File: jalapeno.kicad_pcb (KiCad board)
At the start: 2 copper layers, 230.1 x 77.6 mm, 187 parts, among them IC1 ATMEGA32U4-AU, J1 USB_B, J2 AVR-ISP-6, J3 Conn_01x04, K1 esc, K10 o, K11 p, K12 back, K13 tab, K14 a, K15 s, K16 d, K17 f, K18 g, K19 h, K2 q, K20 j, K21 k, K22 l, K23 ;, K24 caps, K25 caps, K26 z, K27 x, K28 c, K29 v, K3 w, K30 b, K31 n, K32 m, K33 ,, K33_1 ,, K34 ., K34_1 ., K35 ctrl, K36 gui, K37 alt, K37_1 alt, K38 space, K38_1 space, K39 alt, K39_1 gui, K4 e, K40 gui, K41 ctrl, K42 KEYSW, K5 r, K6 t, K7 y, K8 u, K9 i, Q1 MMBT2222ALT3G, SW1 SW_PUSH, U1 MDBT40, U2 SPX3819M5-L-3-3, U3 MCP73831T-2ACI/OT, Y1 XTAL_GND

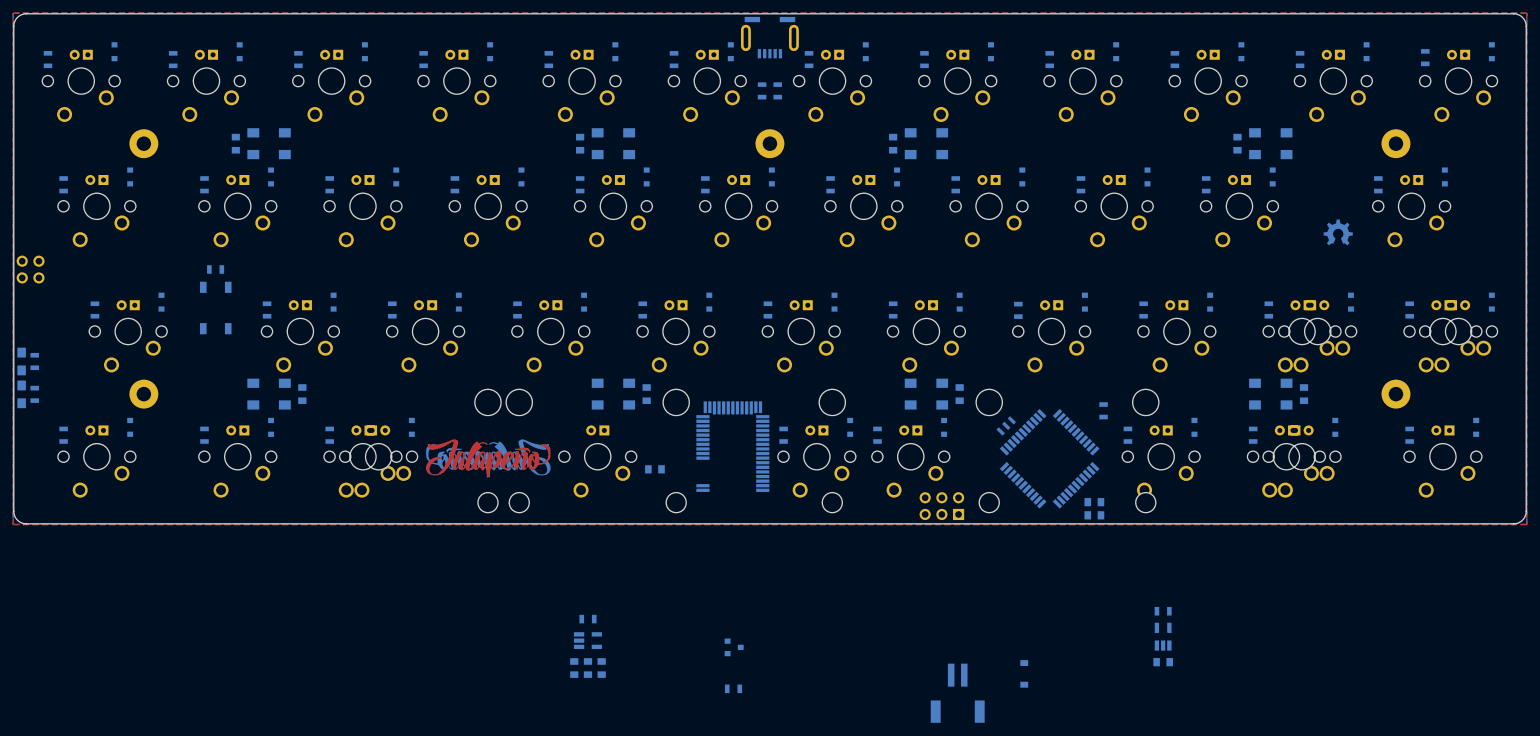
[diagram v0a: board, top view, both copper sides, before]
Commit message: routing + plate
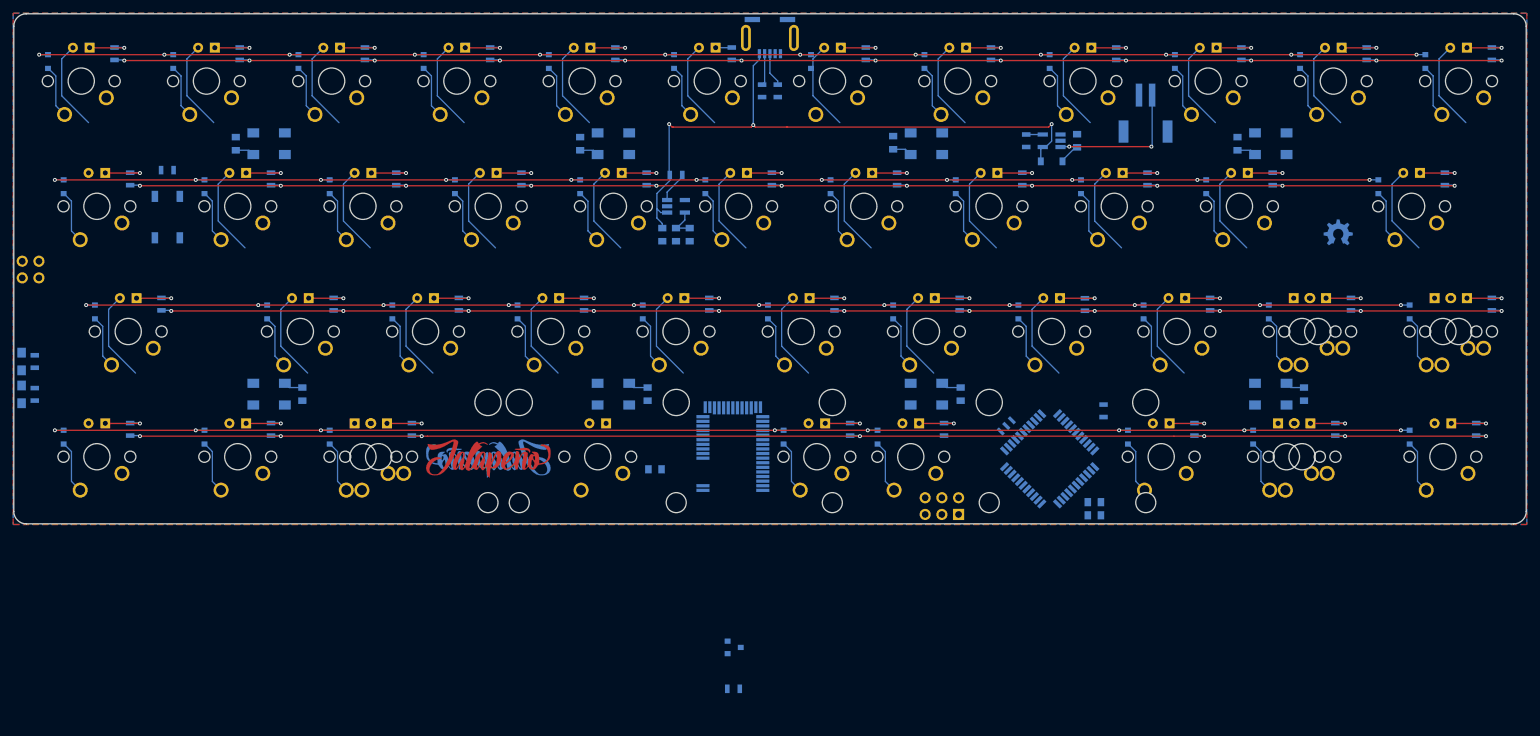
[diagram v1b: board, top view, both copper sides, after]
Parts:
- H1, H2, H3, H4, H6: footprint Mounting_Holes:MountingHole_2.2mm_M2_Pad -> Jalapeno:NOOP
- K33, K37_1: footprint Jalapeno:CHERRY_PCB_125H_LED_REVERSED -> Jalapeno:CHERRY_PCB_125H_LED
- K33_1, K37: footprint Jalapeno:CHERRY_PCB_100H_LED -> Jalapeno:CHERRY_PCB_100H_LED_REVERSED
- K34, K39_1: footprint Jalapeno:CHERRY_PCB_100H_LED_REVERSED -> Jalapeno:CHERRY_PCB_100H_LED
- K34_1, K39: footprint Jalapeno:CHERRY_PCB_125H_LED -> Jalapeno:CHERRY_PCB_125H_LED_REVERSED
- moved JST1 92.8 mm to (204.8, 42.7)
- moved C3 80.4 mm to (194.4, 42.4), turned to 90 degrees
- moved DB1 78.1 mm to (190.5, 45.5), turned to 0 degrees
- moved U3 77.3 mm to (190.5, 42.4), turned to 180 degrees
- moved R3 74.6 mm to (186.6, 42.4), turned to 90 degrees
- moved R6 68.9 mm to (133.3, 47.6)
- moved U2 67.4 mm to (133.3, 52.4)
- moved C5 67.3 mm to (133.3, 56.7)
- moved C6 67.3 mm to (131.3, 56.7)
- moved C7 67.3 mm to (135.4, 56.7)
- moved R7 16.8 mm to (56.0, 46.9), turned to 0 degrees
- moved SW1 15.7 mm to (56.0, 54.0), turned to 270 degrees
- moved D33 12.6 mm to (223.5, 68.5)
- moved D34 12.6 mm to (245.0, 68.5)
- moved D39 12.6 mm to (221.2, 87.5)
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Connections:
- K1 pad 1: COL_1 -> Net-(D1-Pad2)
- K1 pad 2: Net-(D1-Pad2) -> COL_1
- K10 pad 1: COL_10 -> Net-(D10-Pad2)
- K10 pad 2: Net-(D10-Pad2) -> COL_10
- K11 pad 1: COL_11 -> Net-(D11-Pad2)
- K11 pad 2: Net-(D11-Pad2) -> COL_11
- K12 pad 1: COL_12 -> Net-(D12-Pad2)
- K12 pad 2: Net-(D12-Pad2) -> COL_12
- K13 pad 1: COL_1 -> Net-(D13-Pad2)
- K13 pad 2: Net-(D13-Pad2) -> COL_1
- K14 pad 1: COL_2 -> Net-(D14-Pad2)
- K14 pad 2: Net-(D14-Pad2) -> COL_2
- K15 pad 1: COL_3 -> Net-(D15-Pad2)
- K15 pad 2: Net-(D15-Pad2) -> COL_3
- K16 pad 1: COL_4 -> Net-(D16-Pad2)
- K16 pad 2: Net-(D16-Pad2) -> COL_4
- K17 pad 1: COL_5 -> Net-(D17-Pad2)
- K17 pad 2: Net-(D17-Pad2) -> COL_5
- K18 pad 1: COL_6 -> Net-(D18-Pad2)
- K18 pad 2: Net-(D18-Pad2) -> COL_6
- K19 pad 1: COL_7 -> Net-(D19-Pad2)
- K19 pad 2: Net-(D19-Pad2) -> COL_7
- K2 pad 1: COL_2 -> Net-(D2-Pad2)
- K2 pad 2: Net-(D2-Pad2) -> COL_2
- K20 pad 1: COL_8 -> Net-(D20-Pad2)
- K20 pad 2: Net-(D20-Pad2) -> COL_8
- K21 pad 1: COL_9 -> Net-(D21-Pad2)
- K21 pad 2: Net-(D21-Pad2) -> COL_9
- K22 pad 1: COL_10 -> Net-(D22-Pad2)
- K22 pad 2: Net-(D22-Pad2) -> COL_10
- K23 pad 1: COL_11 -> Net-(D23-Pad2)
- K23 pad 2: Net-(D23-Pad2) -> COL_11
- K24 pad 1: COL_1 -> Net-(D24-Pad2)
- K24 pad 2: Net-(D24-Pad2) -> COL_1
- K25 pad 1: COL_2 -> Net-(D25-Pad2)
- K25 pad 2: Net-(D25-Pad2) -> COL_2
- K26 pad 1: COL_3 -> Net-(D26-Pad2)
- K26 pad 2: Net-(D26-Pad2) -> COL_3
- K27 pad 1: COL_4 -> Net-(D27-Pad2)
- K27 pad 2: Net-(D27-Pad2) -> COL_4
- K28 pad 1: COL_5 -> Net-(D28-Pad2)
- K28 pad 2: Net-(D28-Pad2) -> COL_5
- K29 pad 1: COL_6 -> Net-(D29-Pad2)
- K29 pad 2: Net-(D29-Pad2) -> COL_6
- K3 pad 1: COL_3 -> Net-(D3-Pad2)
- K3 pad 2: Net-(D3-Pad2) -> COL_3
- K30 pad 1: COL_7 -> Net-(D30-Pad2)
- K30 pad 2: Net-(D30-Pad2) -> COL_7
- K31 pad 1: COL_8 -> Net-(D31-Pad2)
- K31 pad 2: Net-(D31-Pad2) -> COL_8
- K32 pad 1: COL_9 -> Net-(D32-Pad2)
- K32 pad 2: Net-(D32-Pad2) -> COL_9
- K33 pad 1: COL_10 -> Net-(D33-Pad2)
- K33 pad 2: Net-(D33-Pad2) -> COL_10
- K33_1 pad 1: COL_10 -> Net-(D33-Pad2)
- K33_1 pad 2: Net-(D33-Pad2) -> COL_10
- K34 pad 1: COL_11 -> Net-(D34-Pad2)
- K34 pad 2: Net-(D34-Pad2) -> COL_11
- K34_1 pad 1: COL_11 -> Net-(D34-Pad2)
- K34_1 pad 2: Net-(D34-Pad2) -> COL_11
- K35 pad 1: COL_1 -> Net-(D35-Pad2)
- K35 pad 2: Net-(D35-Pad2) -> COL_1
- K36 pad 1: COL_2 -> Net-(D36-Pad2)
- K36 pad 2: Net-(D36-Pad2) -> COL_2
- K37 pad 1: COL_3 -> Net-(D37-Pad2)
- K37 pad 2: Net-(D37-Pad2) -> COL_3
- K37_1 pad 1: COL_3 -> Net-(D37-Pad2)
- K37_1 pad 2: Net-(D37-Pad2) -> COL_3
- K38 pad 1: COL_4 -> Net-(D38-Pad2)
- K38 pad 2: Net-(D38-Pad2) -> COL_4
- K38_1 pad 1: COL_4 -> Net-(D38-Pad2)
- K38_1 pad 2: Net-(D38-Pad2) -> COL_4
- K39 pad 1: COL_5 -> Net-(D39-Pad2)
- K39 pad 2: Net-(D39-Pad2) -> COL_5
- K39_1 pad 1: COL_5 -> Net-(D39-Pad2)
- K39_1 pad 2: Net-(D39-Pad2) -> COL_5
- K4 pad 1: COL_4 -> Net-(D4-Pad2)
- K4 pad 2: Net-(D4-Pad2) -> COL_4
- K40 pad 1: COL_6 -> Net-(D40-Pad2)
- K40 pad 2: Net-(D40-Pad2) -> COL_6
- K41 pad 1: COL_7 -> Net-(D41-Pad2)
- K41 pad 2: Net-(D41-Pad2) -> COL_7
- K42 pad 1: COL_8 -> Net-(D42-Pad2)
- K42 pad 2: Net-(D42-Pad2) -> COL_8
- K5 pad 1: COL_5 -> Net-(D5-Pad2)
- K5 pad 2: Net-(D5-Pad2) -> COL_5
- K6 pad 1: COL_6 -> Net-(D6-Pad2)
- K6 pad 2: Net-(D6-Pad2) -> COL_6
- K7 pad 1: COL_7 -> Net-(D7-Pad2)
- K7 pad 2: Net-(D7-Pad2) -> COL_7
- K8 pad 1: COL_8 -> Net-(D8-Pad2)
- K8 pad 2: Net-(D8-Pad2) -> COL_8
- K9 pad 1: COL_9 -> Net-(D9-Pad2)
- K9 pad 2: Net-(D9-Pad2) -> COL_9
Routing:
- net LEDGND: track 0.00 -> 879.6 mm, vias 0 -> 41
- net +3V3: track 0.00 -> 456.6 mm
- net ROW_1: track 0.00 -> 226.0 mm, vias 0 -> 12
- net ROW_4: track 0.00 -> 215.7 mm, vias 0 -> 8
- net ROW_2: track 0.00 -> 214.8 mm, vias 0 -> 11
- net ROW_3: track 0.00 -> 214.8 mm, vias 0 -> 11
- net VBUS: track 0.00 -> 95.6 mm, vias 0 -> 3
- net +BATT: track 0.00 -> 26.2 mm, vias 0 -> 2
- net Net-(D12-Pad2): track 0.00 -> 8.08 mm
- net Net-(D39-Pad2): track 0.00 -> 8.03 mm
- net Net-(D23-Pad2): track 0.00 -> 8.03 mm
- net Net-(D6-Pad2): track 0.00 -> 8.03 mm
- net Net-(D11-Pad2): track 0.00 -> 8.03 mm
- net Net-(D33-Pad2): track 0.00 -> 8.03 mm
- net Net-(D28-Pad2): track 0.00 -> 8.03 mm
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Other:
- net class Default: clearance 0.15 -> 0.13; trace_width 0.15 -> 0.2
- rule trace_clearance: 0.15 -> 0.13
- rule trace_min: 0.15 -> 0.13
